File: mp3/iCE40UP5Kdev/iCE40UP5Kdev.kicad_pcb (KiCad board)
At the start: 2 copper layers, 21.8 x 51.9 mm, 57 parts, among them J1 USB4105-GF-A, J2 Left, J3 Right, J4 Conn_02x03_Counter_Clockwise, U1 W25Q32JV, U2 MIC5365-1-2YD5, U3 MIC5318-3-3YD5, U4 ICE40UP5K-SG48ITR, X1 IQXO-791

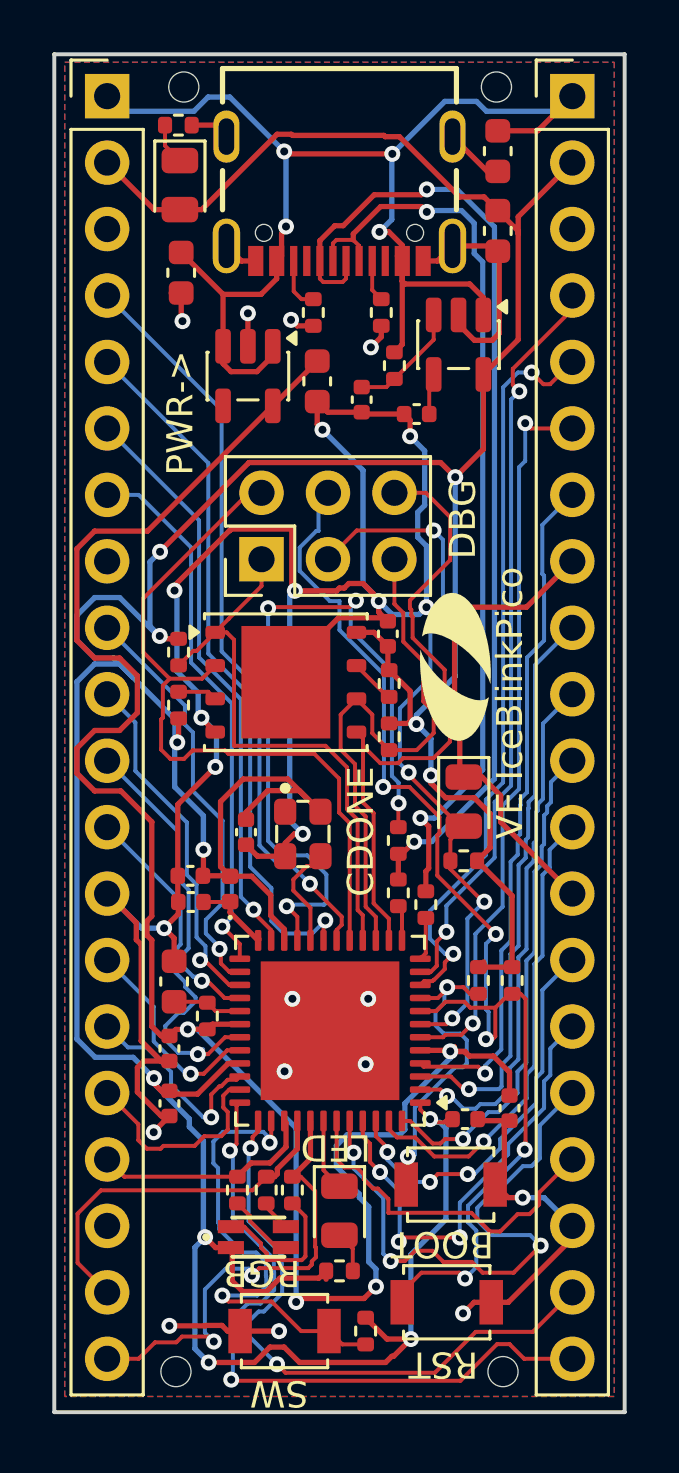
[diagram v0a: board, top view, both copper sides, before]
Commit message: fix gaps in power pour
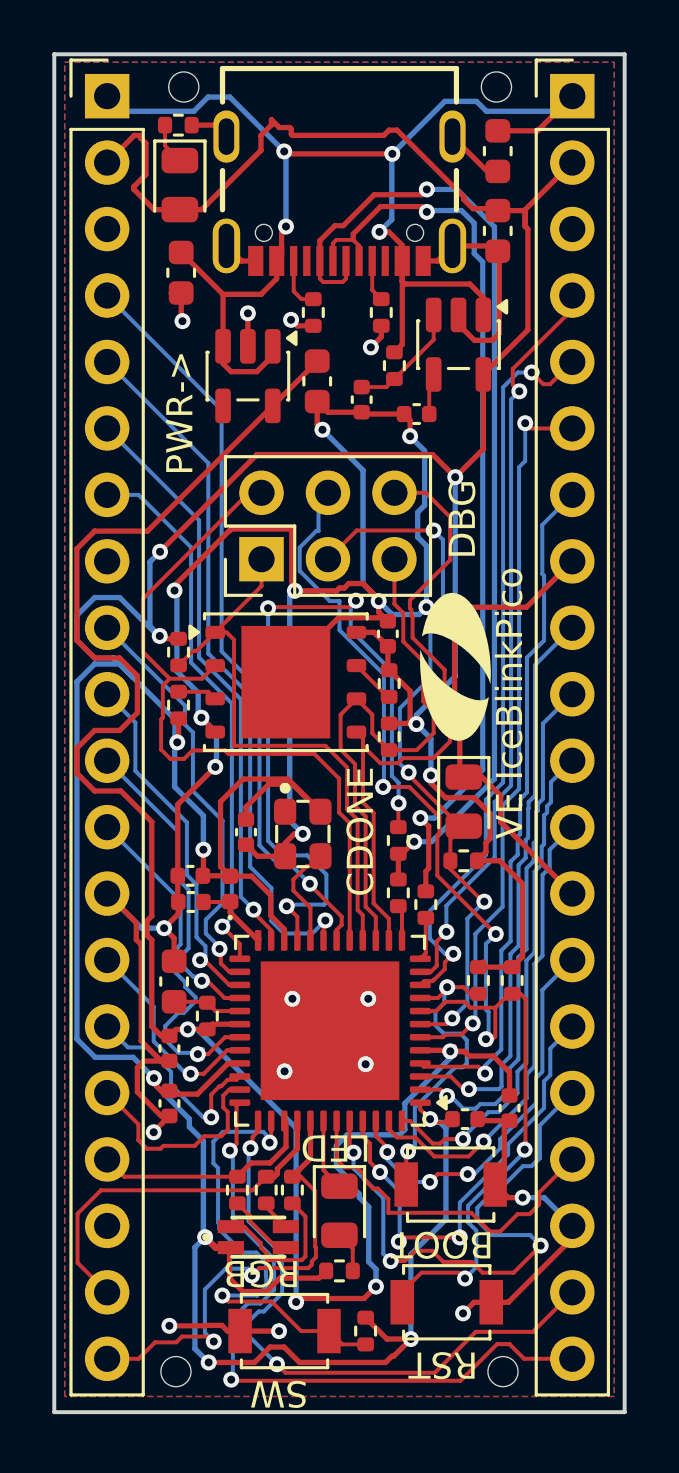
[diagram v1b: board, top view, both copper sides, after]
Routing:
- net +3V3: track 178.8 -> 184.8 mm
